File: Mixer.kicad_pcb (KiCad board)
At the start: 2 copper layers, 60 x 100 mm, 48 parts, among them J1 Audio-Jack-2_Switch, J2 Conn_02x05_Odd_Even, J3 Audio-Jack-2_Switch, J4 Audio-Jack-2_Switch, J5 Audio-Jack-2_Switch, J6 Audio-Jack-2_Switch, J7 Audio-Jack-2_Switch, U1 TL074

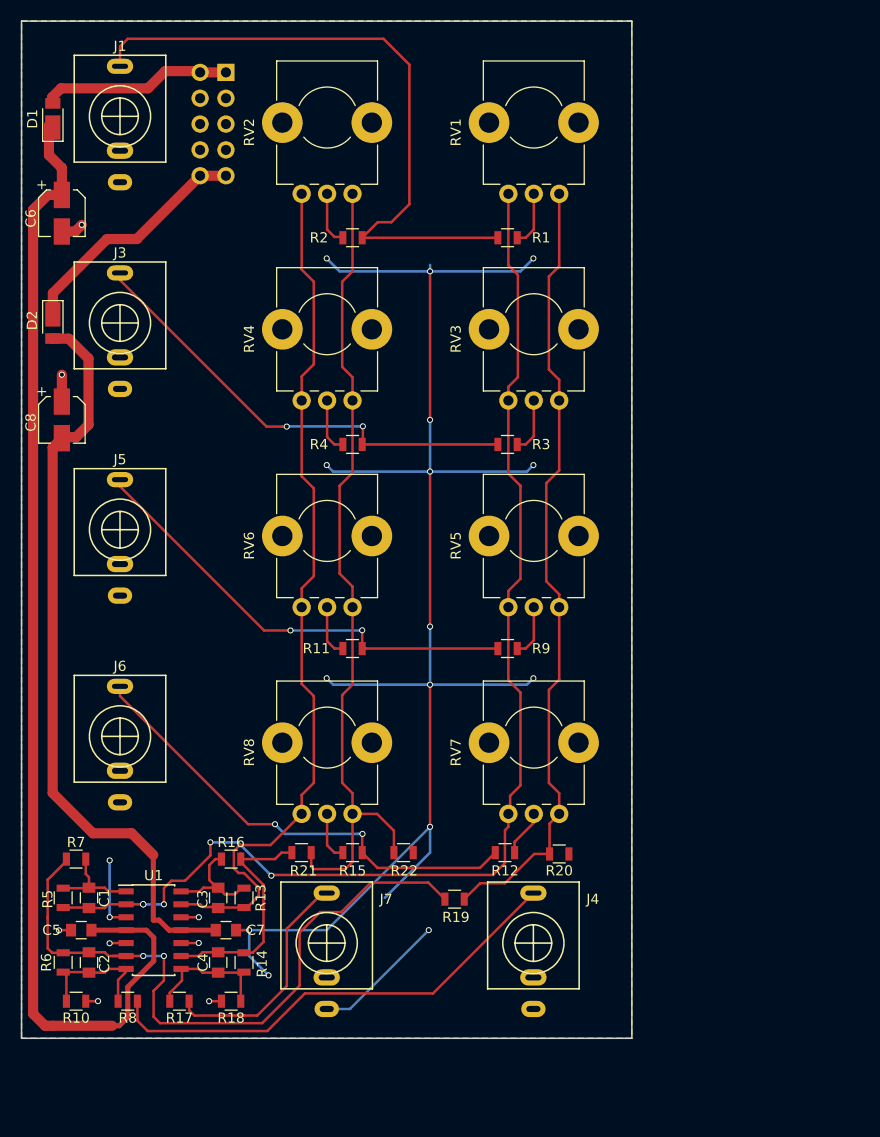
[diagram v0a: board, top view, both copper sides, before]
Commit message: This is revision B of the board.
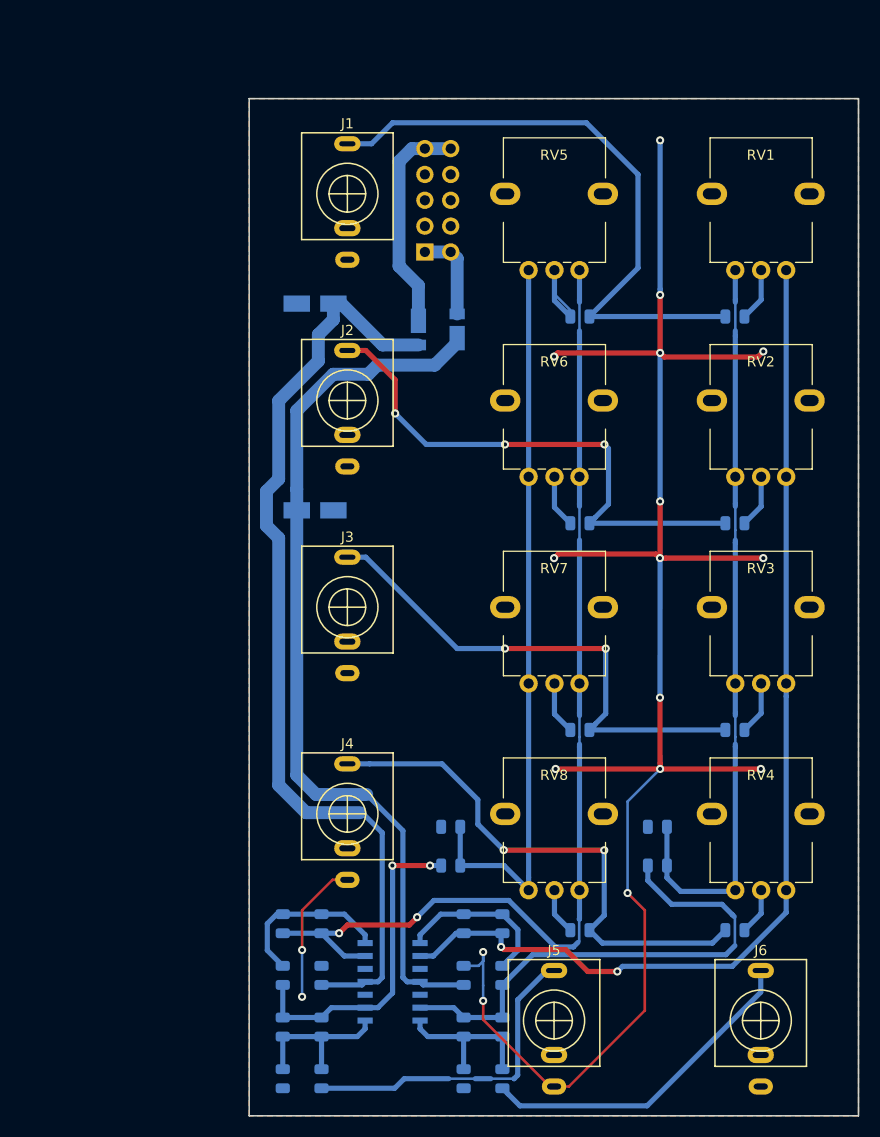
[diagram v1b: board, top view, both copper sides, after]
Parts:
- C1, C2, C3, C4, C5, C7: footprint Capacitors_SMD:C_0805 -> Capacitor_SMD:C_0805_2012Metric; moved to B.Cu
- C6, C8: footprint Capacitors_SMD:CP_Elec_4x5.8 -> Capacitor_SMD:CP_Elec_4x5.8; moved to B.Cu
- D1, D2: footprint Diodes_SMD:D_PowerDI-123 -> Diode_SMD:D_PowerDI-123; moved to B.Cu
- J1, J3, J4, J5, J6: value Audio-Jack-2_Switch -> AudioJack2_Ground_Switch; footprint DTD:PJ398SM -> Local:PJ398SM
- J2: value Conn_02x05_Odd_Even -> AudioJack2_Ground_Switch; footprint Pin_Headers:Pin_Header_Straight_2x05_Pitch2.54mm -> Local:PJ398SM; moved to F.Cu
- J7: value Audio-Jack-2_Switch -> Conn_02x05_Odd_Even; footprint DTD:PJ398SM -> Connector_PinHeader_2.54mm:PinHeader_2x05_P2.54mm_Vertical; moved to B.Cu
- R1, R10, R11, R12, R13, R14, R15, R16, R17, R18, R19, R2, R20, R21, R22, R3, R4, R5, R6, R7, R8, R9: footprint Resistors_SMD:R_0805 -> Resistor_SMD:R_0805_2012Metric; moved to B.Cu
- RV1, RV2, RV3, RV4, RV5, RV6, RV7, RV8: value 47k -> 50k; footprint Potentiometers:Potentiometer_Alps_RK09K_Horizontal -> Local:AlpsRK09K
- U1: footprint Housings_SOIC:SOIC-14_3.9x8.7mm_Pitch1.27mm -> Package_SO:SOIC-14_3.9x8.7mm_P1.27mm; moved to B.Cu
- moved J6 68.9 mm to (139.2, 142.2)
- moved J7 68.6 mm to (106.2, 66.7)
- moved J5 64.4 mm to (118.9, 142.2)
- moved RV4 57.1 mm to (139.2, 121.9), turned to 0 degrees
- moved RV2 45.0 mm to (139.2, 81.3), turned to 0 degrees
- moved D1 44.8 mm to (109.3, 74.3)
- moved RV5 40.6 mm to (118.9, 61.0), turned to 0 degrees
- moved R11 38.4 mm to (136.7, 113.7), turned to 180 degrees
- moved R2 38.4 mm to (136.7, 73.0), turned to 180 degrees
- moved R4 38.4 mm to (136.7, 93.3), turned to 180 degrees
- moved C6 38.4 mm to (95.4, 92.1), turned to 0 degrees
- moved R15 38.4 mm to (136.7, 133.3), turned to 180 degrees
- moved C5 37.9 mm to (110.0, 137.8), turned to 90 degrees
- moved D2 35.9 mm to (105.5, 74.3)
- moved J3 35.8 mm to (98.6, 101.6)
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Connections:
- J7 pad 1: Net-(J7-Pad1) -> Net-(D1-Pad2)
- J7 pad 2: GND -> Net-(D1-Pad2)
- J7 pad 3: Net-(J7-Pad3) -> GND
- R1 pad 2: Net-(J1-Pad1) -> Net-(J1-PadT)
- R11 pad 2: Net-(J5-Pad1) -> Net-(J3-PadT)
- R12 pad 2: Net-(J6-Pad1) -> Net-(J4-PadT)
- R15 pad 2: Net-(J6-Pad1) -> Net-(J4-PadT)
- R17 pad 1: Net-(J7-Pad1) -> Net-(J6-PadT)
- R2 pad 2: Net-(J1-Pad1) -> Net-(J1-PadT)
- R3 pad 2: Net-(J3-Pad1) -> Net-(J2-PadT)
- R4 pad 2: Net-(J3-Pad1) -> Net-(J2-PadT)
- R8 pad 1: Net-(J4-Pad1) -> Net-(J5-PadT)
- R9 pad 2: Net-(J5-Pad1) -> Net-(J3-PadT)
- RV1 pad 1: Net-(R19-Pad2) -> Net-(C3-Pad2)
- RV1 pad 2: Net-(R1-Pad1) -> Net-(R2-Pad1)
- RV1 pad 3: Net-(C1-Pad2) -> Net-(R21-Pad2)
- RV2 pad 1: Net-(R21-Pad2) -> Net-(C3-Pad2)
- RV2 pad 2: Net-(R2-Pad1) -> Net-(R4-Pad1)
- RV2 pad 3: Net-(C3-Pad2) -> Net-(R21-Pad2)
- RV3 pad 1: Net-(R19-Pad2) -> Net-(C3-Pad2)
- RV3 pad 2: Net-(R3-Pad1) -> Net-(R11-Pad1)
- RV3 pad 3: Net-(C1-Pad2) -> Net-(R21-Pad2)
- RV4 pad 1: Net-(R21-Pad2) -> Net-(C3-Pad2)
- RV4 pad 2: Net-(R4-Pad1) -> Net-(R15-Pad1)
- RV4 pad 3: Net-(C3-Pad2) -> Net-(R21-Pad2)
- RV5 pad 1: Net-(R19-Pad2) -> Net-(C1-Pad2)
- RV5 pad 2: Net-(R9-Pad1) -> Net-(R1-Pad1)
- RV5 pad 3: Net-(C1-Pad2) -> Net-(R19-Pad2)
- RV6 pad 1: Net-(R21-Pad2) -> Net-(C1-Pad2)
- RV6 pad 2: Net-(R11-Pad1) -> Net-(R3-Pad1)
- RV6 pad 3: Net-(C3-Pad2) -> Net-(R19-Pad2)
- RV7 pad 1: Net-(R19-Pad2) -> Net-(C1-Pad2)
- RV7 pad 2: Net-(R12-Pad1) -> Net-(R9-Pad1)
- RV7 pad 3: Net-(C1-Pad2) -> Net-(R19-Pad2)
- RV8 pad 1: Net-(R21-Pad2) -> Net-(C1-Pad2)
- RV8 pad 2: Net-(R15-Pad1) -> Net-(R12-Pad1)
- RV8 pad 3: Net-(C3-Pad2) -> Net-(R19-Pad2)
- U1 pad 1: Net-(C1-Pad1) -> Net-(C3-Pad1)
- U1 pad 13: Net-(C3-Pad2) -> Net-(C1-Pad2)
- U1 pad 14: Net-(C3-Pad1) -> Net-(C1-Pad1)
- U1 pad 2: Net-(C1-Pad2) -> Net-(C3-Pad2)
- U1 pad 6: Net-(C2-Pad2) -> Net-(C4-Pad2)
- U1 pad 7: Net-(C2-Pad1) -> Net-(C4-Pad1)
- U1 pad 8: Net-(C4-Pad1) -> Net-(C2-Pad1)
- U1 pad 9: Net-(C4-Pad2) -> Net-(C2-Pad2)
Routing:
- net Net-(J2-PadT): track 0.00 -> 66.8 mm, vias 0 -> 3
- net Net-(J1-Pad1): track 64.8 -> 0.00 mm
- net Net-(J1-PadT): track 0.00 -> 60.8 mm
- net Net-(J4-PadT): track 0.00 -> 53.1 mm, vias 0 -> 2
- net Net-(J3-PadT): track 0.00 -> 51.2 mm, vias 0 -> 2
- net Net-(J3-Pad1): track 47.1 -> 0.00 mm, vias 2 -> 0
- net Net-(J4-Pad1): track 46.9 -> 0.00 mm
- net Net-(J6-Pad1): track 46.7 -> 0.00 mm, vias 2 -> 0
- net Net-(J5-Pad1): track 45.8 -> 0.00 mm, vias 2 -> 0
- net Net-(C2-Pad2): track 67.7 -> 32.3 mm
- net Net-(J5-PadT): track 0.00 -> 33.5 mm
- net Net-(J6-PadT): track 0.00 -> 32.9 mm
- net +12VA: track 115.3 -> 88.2 mm
- net Net-(C4-Pad2): track 23.6 -> 50.6 mm
- net Net-(J7-Pad1): track 22.9 -> 0.00 mm
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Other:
- board size 60 x 100 mm -> 59.9 x 100 mm
- net class Default: clearance 0.2 -> 0.254; trace_width 0.25 -> 0.254; via_dia 0.6 -> 0.8
- rule trace_clearance: 0.2 -> 0.254
- board text added: "Mixer / Attenuverter"
- board text added: "Rev B"
- board text removed: "+12"
- board text removed: "-12"
- board text removed: "Modular Mixer, Rev B"
